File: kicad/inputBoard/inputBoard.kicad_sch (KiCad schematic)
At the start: 0 parts

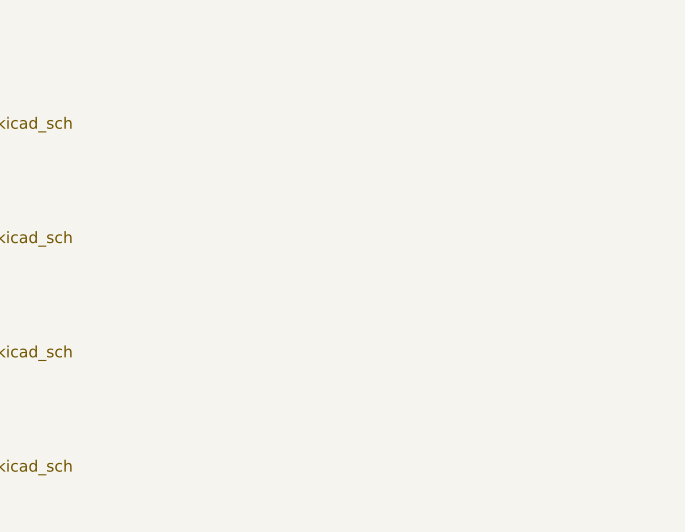
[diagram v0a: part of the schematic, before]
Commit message: finish main input board
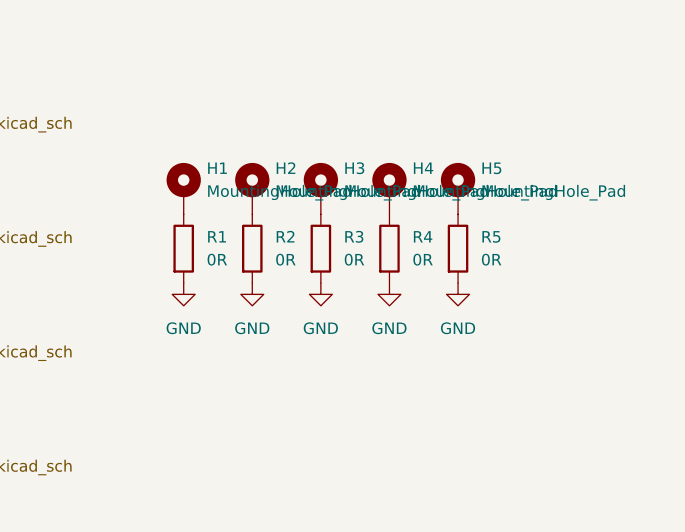
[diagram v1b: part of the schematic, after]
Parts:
- added H1, H2, H3, H4, H5: MountingHole_Pad, MountingHole:MountingHole_2.2mm_M2_DIN965_Pad, symbol Mechanical:MountingHole_Pad
- added R1, R2, R3, R4, R5: 0R, Resistor_SMD:R_1206_3216Metric_Pad1.30x1.75mm_HandSolder, symbol Device:R
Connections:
- new net: H2.1, R2.1
- new net: H5.1, R5.1
- new net: H3.1, R3.1
- new net: H1.1, R1.1
- new net: H4.1, R4.1
- new net GND: R1.2, R2.2, R3.2, R4.2, R5.2
